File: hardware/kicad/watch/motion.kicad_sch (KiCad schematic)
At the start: 9 parts, among them IC1 LSM6DSV80XTR, IC4 ICU-10201, U4 BMM350

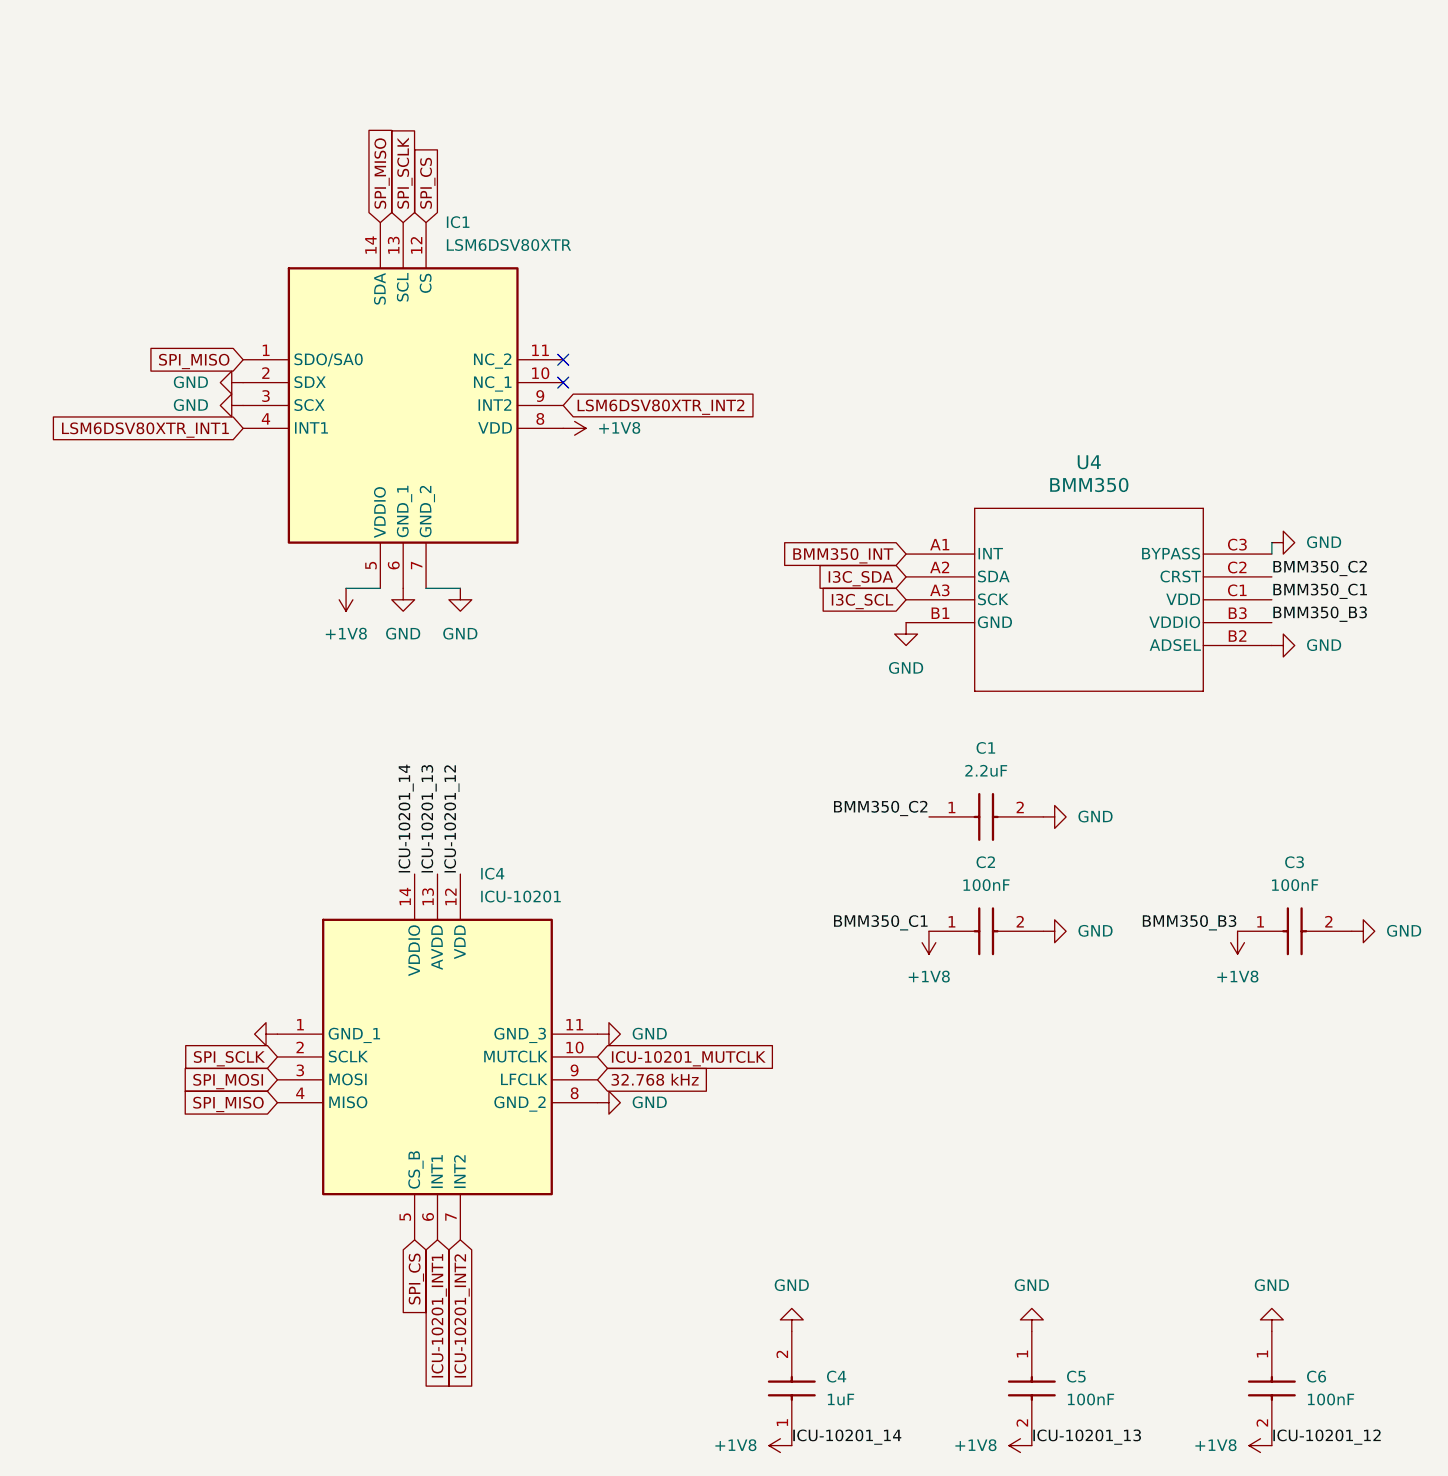
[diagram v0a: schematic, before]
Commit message: fah
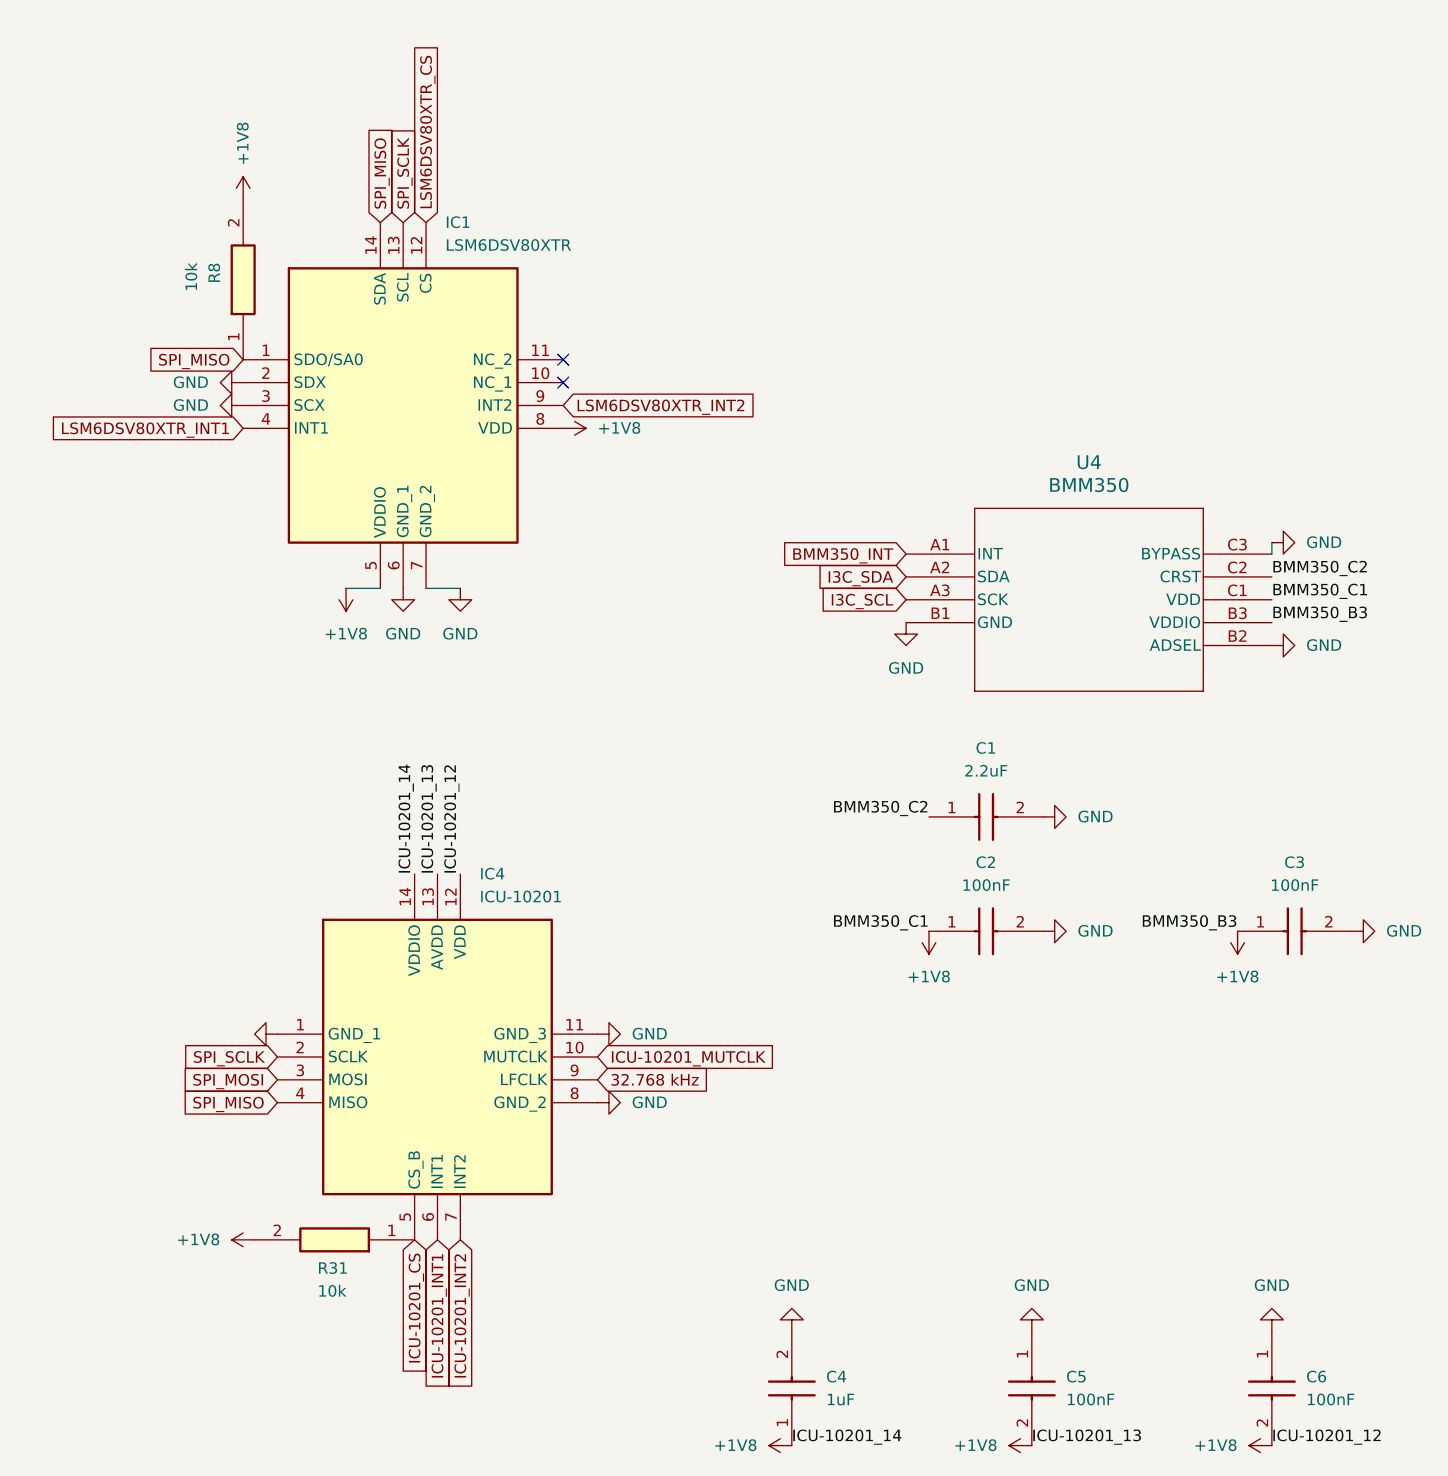
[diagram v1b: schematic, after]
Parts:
- added R31, R8: 10k, Footprints:ERJS02_U02__0402_, symbol Symbols:ERJU02F1002X
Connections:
- net +1V8: now also R31.2, R8.2
- net SPI_MISO: now also R8.1
- net SPI_CS renamed ICU-10201_CS
- net ICU-10201_CS: now also R31.1; no longer IC1.12 (CS)
- new net LSM6DSV80XTR_CS: IC1.12 (CS)
